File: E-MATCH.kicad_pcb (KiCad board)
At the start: 4 copper layers, 63.8 x 63 mm, 26 parts, among them IC1 NCV81071BZR2G, IC2 NCV81071BZR2G, J1 691210910002, J2 691210910002, J3 691210910002, J4 691210910002, J5 DC Jack, Q1 AOSP36326C, Q2 AOSP36326C, Q3 AOSP36326C, Q4 AOSP36326C, U1 TMCS1108A2UQDR

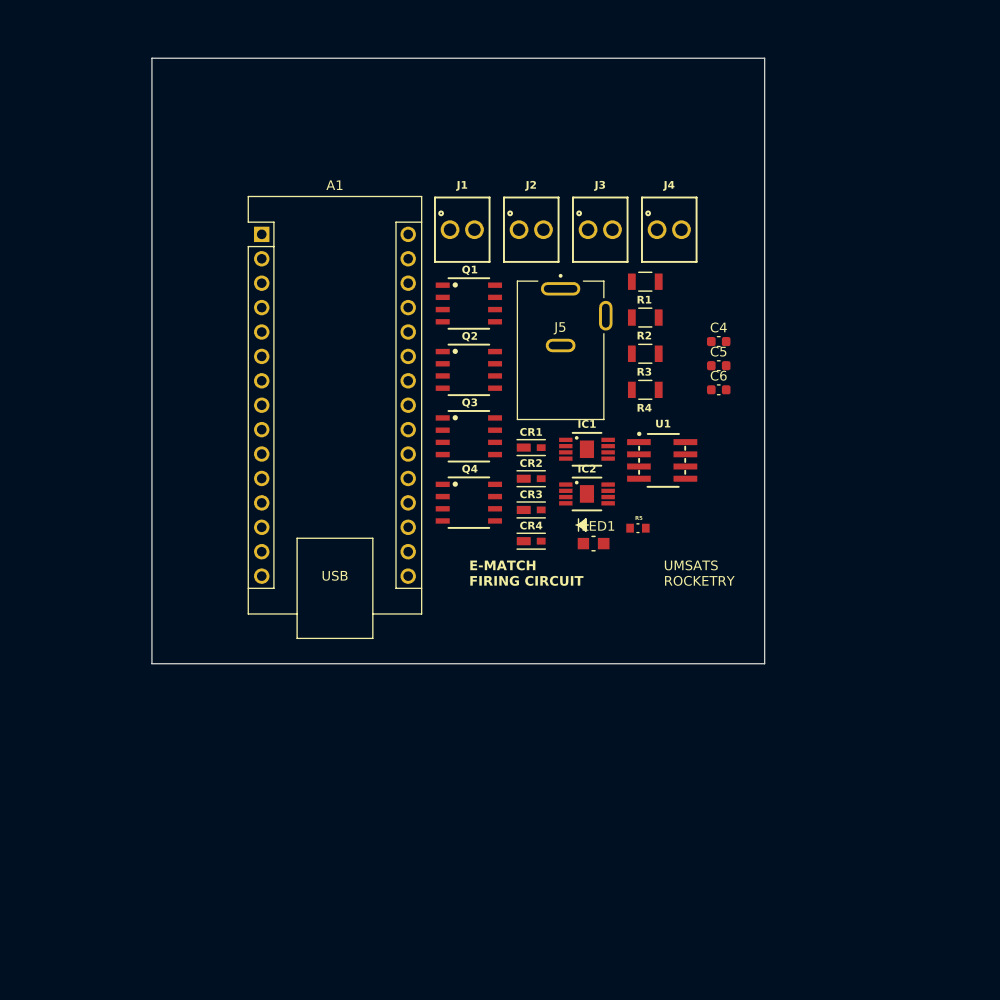
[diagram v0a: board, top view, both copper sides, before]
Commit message: some changes
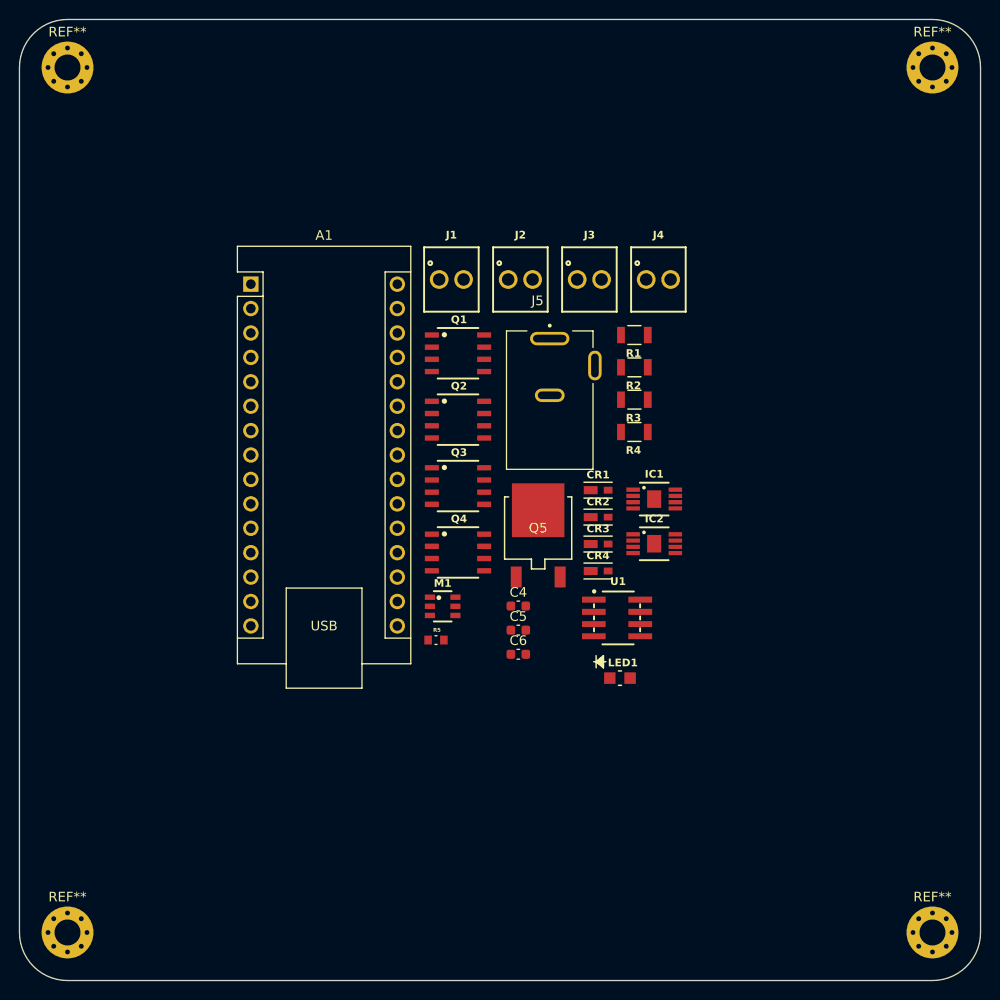
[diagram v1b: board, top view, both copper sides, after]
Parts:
- added M1: FDC8878, FDC8878:SuperSot6_SOT-23-6_1P6X2P9_ONS, F.Cu at (145.5, 107.5)
- added Q5: FDD1600N10ALZ, FDD1600N10ALZ:TO252_FDD1600_ONS-L, F.Cu at (155.4, 99.4)
- added REF**: MountingHole_2.7mm_Pad_Via, MountingHole:MountingHole_2.7mm_Pad_Via, F.Cu at (106.5, 141.5)
- added REF**: MountingHole_2.7mm_Pad_Via, MountingHole:MountingHole_2.7mm_Pad_Via, F.Cu at (106.5, 51.5)
- added REF**: MountingHole_2.7mm_Pad_Via, MountingHole:MountingHole_2.7mm_Pad_Via, F.Cu at (196.5, 141.5)
- added REF**: MountingHole_2.7mm_Pad_Via, MountingHole:MountingHole_2.7mm_Pad_Via, F.Cu at (196.5, 51.5)
- moved C4 34.5 mm to (153.4, 107.5)
- moved C5 34.5 mm to (153.4, 110.0)
- moved C6 34.5 mm to (153.4, 112.5)
- moved R5 24.0 mm to (144.8, 111.0)
- moved U1 17.0 mm to (163.6, 108.7)
- moved LED1 14.3 mm to (163.9, 115.0)
- moved IC1 8.71 mm to (167.5, 96.4)
- moved IC2 8.71 mm to (167.5, 101.0)
- moved CR1 8.25 mm to (161.7, 95.4)
- moved CR2 8.03 mm to (161.7, 98.2)
- moved CR3 7.81 mm to (161.7, 101.0)
- moved CR4 7.62 mm to (161.7, 103.9)
- moved R1 5.67 mm to (165.4, 79.3)
- moved A1 5.30 mm to (125.5, 74.0)
- moved J1 5.30 mm to (146.4, 73.5)
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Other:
- board size 63.8 x 63 mm -> 100 x 100 mm
- board text removed: "E-MATCH FIRING CIRCUIT"
- board text removed: "UMSATS ROCKETRY"
